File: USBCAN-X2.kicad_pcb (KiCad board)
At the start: 2 copper layers, 73 x 40.5 mm, 29 parts, among them J1 USB_B, J2 Screw_Terminal_01x08, J3 Conn_01x02_Pin, J4 Conn_02x05_Odd_Even, J5 Conn_01x02_Pin, J6 Conn_01x02_Pin, U1 STM32G491CETx, U2 LM2936-3.3, U3 MCP2542FDxMF, U4 MCP2542FDxMF, Y1 Crystal_Small

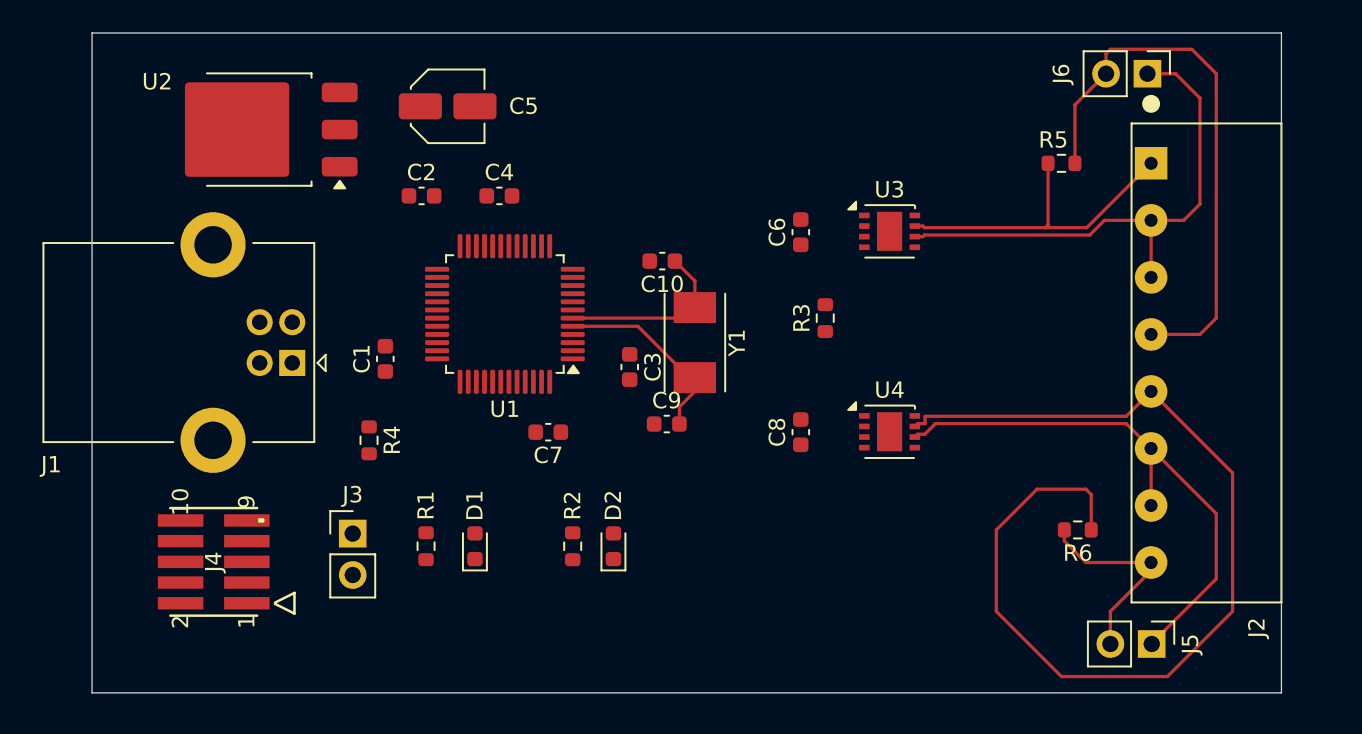
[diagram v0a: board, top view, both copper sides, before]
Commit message: Update
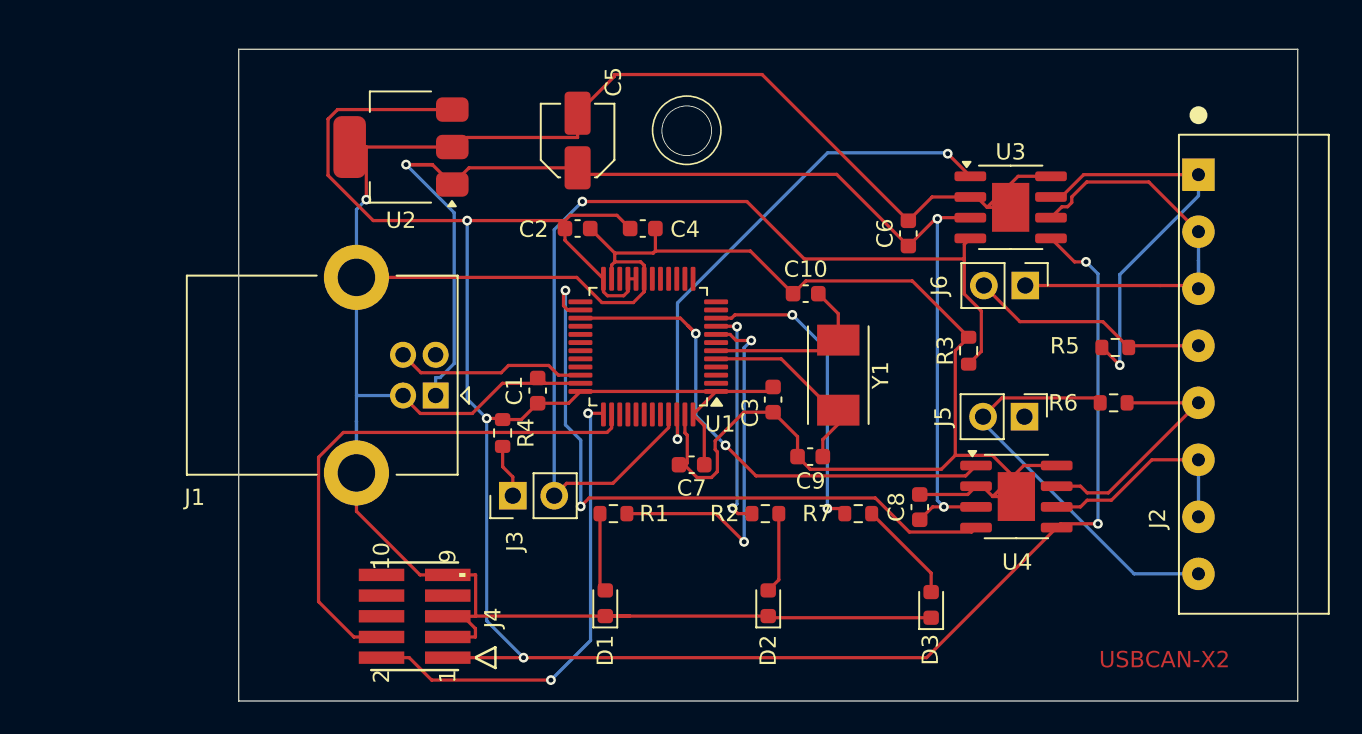
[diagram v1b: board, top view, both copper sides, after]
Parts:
- added D3: LED, LED_SMD:LED_0603_1608Metric, F.Cu at (167.5, 119.1)
- added R7: 330, Resistor_SMD:R_0603_1608Metric, F.Cu at (163.0, 113.5)
- U2: footprint Package_TO_SOT_SMD:TO-252-3_TabPin2 -> Package_TO_SOT_SMD:SOT-223-3_TabPin2
- U3, U4: footprint Package_DFN_QFN:DFN-8-1EP_3x3mm_P0.65mm_EP1.55x2.4mm -> Package_SO:SOIC-8-1EP_3.9x4.9mm_P1.27mm_EP2.29x3mm
- moved J5 16.0 mm to (173.2, 107.5)
- moved J6 15.0 mm to (173.3, 99.5)
- moved J4 12.8 mm to (135.8, 119.8)
- moved R2 12.0 mm to (157.3, 113.5), turned to 0 degrees
- moved R5 11.8 mm to (178.8, 103.3)
- moved R1 11.7 mm to (148.0, 113.5), turned to 180 degrees
- moved D2 10.1 mm to (157.5, 119.0)
- moved J3 10.1 mm to (141.8, 112.4), turned to 90 degrees
- moved C2 9.78 mm to (145.8, 96.0)
- moved C1 9.55 mm to (143.3, 106.0)
- moved C10 9.02 mm to (159.8, 100.0)
- moved C3 9.02 mm to (157.8, 106.5)
- moved C4 9.02 mm to (149.8, 96.0)
- moved C7 9.02 mm to (152.8, 110.5)
- moved J1 9.02 mm to (137.1, 106.2)
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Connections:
- U1 pad 10: unconnected-(U1-PA2-Pad10) -> /LED_PA2
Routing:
- net GND: track 0.00 -> 244.7 mm, vias 0 -> 1
- net 3.3V: track 0.00 -> 154.4 mm, vias 0 -> 5
- net 5V: track 0.00 -> 79.7 mm, vias 0 -> 3
- net CAN1_RX: track 0.00 -> 62.3 mm, vias 0 -> 1
- net CAN2_P: track 63.2 -> 15.6 mm
- net CAN2_RX: track 0.00 -> 41.4 mm, vias 0 -> 2
- net SWDCLK: track 0.00 -> 33.6 mm
- net CAN2_TX: track 0.00 -> 32.9 mm, vias 0 -> 2
- net CAN1_TX: track 0.00 -> 32.1 mm, vias 0 -> 2
- net SWDIO: track 0.00 -> 29.8 mm, vias 0 -> 2
- net /LED_PA0: track 0.00 -> 22.8 mm, vias 0 -> 2
- net CAN2_N: track 34.3 -> 14.4 mm
- net Net-(J2-Pin_4): track 34.4 -> 14.8 mm
- net /LED_PA2: track 0.00 -> 18.7 mm, vias 0 -> 2
- net /LED_PA1: track 0.00 -> 13.9 mm, vias 0 -> 2
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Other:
- board size 73 x 40.5 mm -> 65 x 40 mm
- board text added: "USBCAN-X2"
